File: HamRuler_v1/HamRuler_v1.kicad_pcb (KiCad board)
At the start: 2 copper layers, 13 parts, among them J1 Conn_01x03, Q1 BUK7M9R9-60EX, Q2 BUK7M9R9-60EX, U1 AT42QT1011-TSHR, U2 AT42QT1011-TSHR

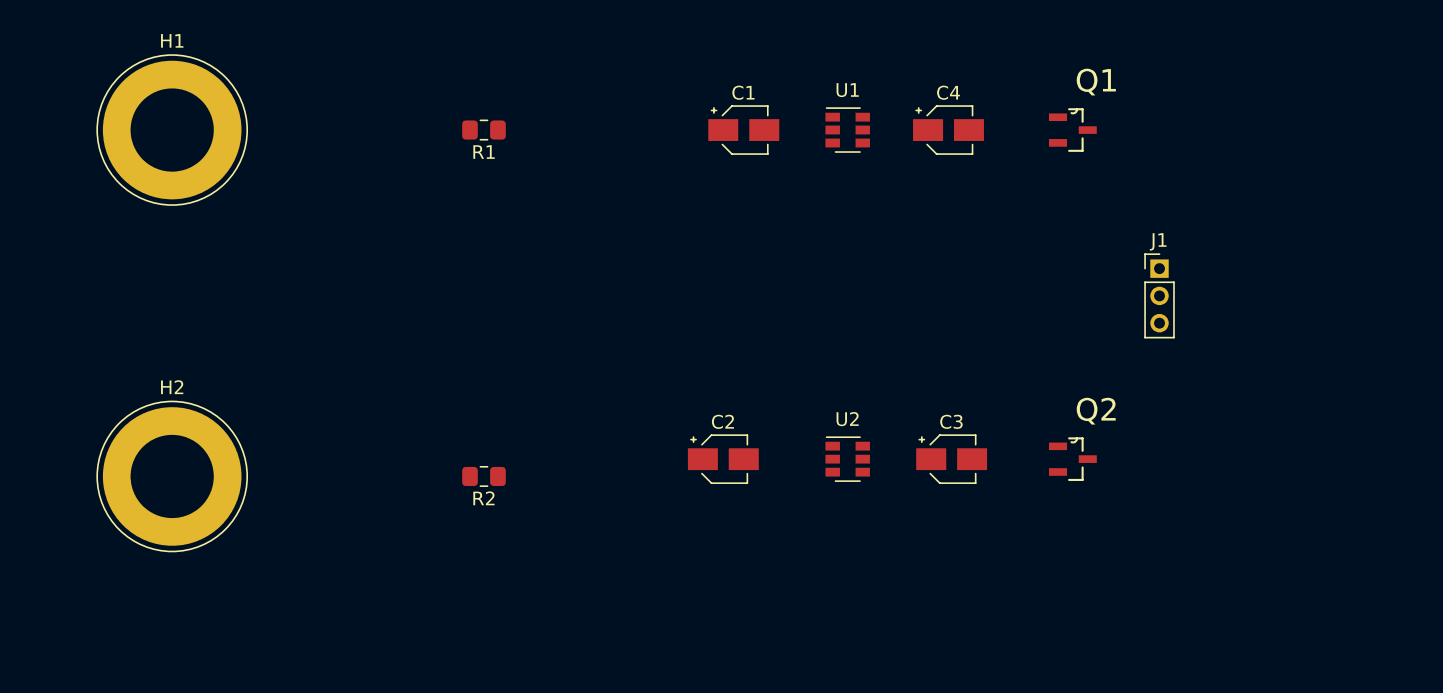
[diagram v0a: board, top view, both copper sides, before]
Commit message: nightly
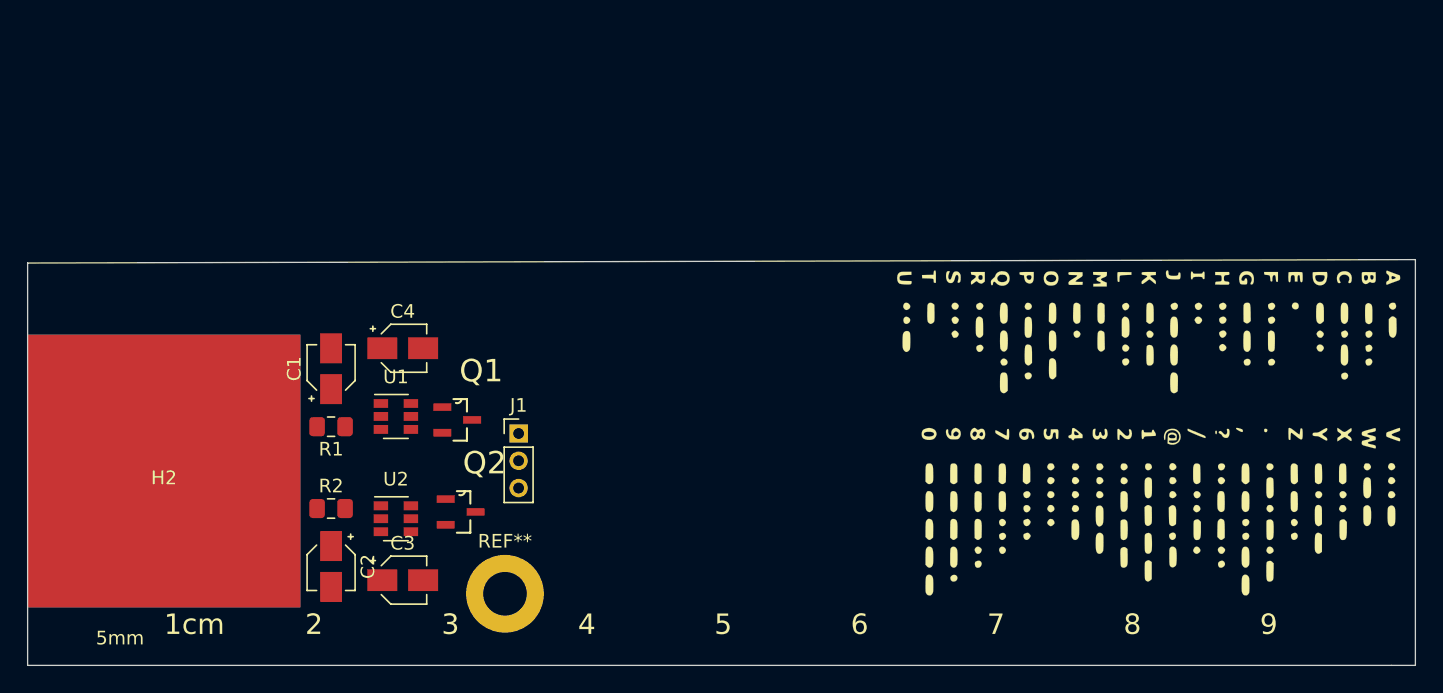
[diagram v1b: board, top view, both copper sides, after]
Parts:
- added G***: LOGO, Resources:morse_code, F.Cu at (110.0, 85.8)
- added REF**: MountingHole_3.2mm_M3_ISO7380_Pad, MountingHole:MountingHole_3.2mm_M3_ISO7380_Pad, F.Cu at (62.5, 97.5)
- added REF**: 4in_ruler, Resources:4in_ruler, B.Cu at (27.5, 73.2)
- added REF**: Metric_Ruler_100mm, Resources:Metric_Ruler_100mm, F.Cu at (27.5, 102.8)
- H1: footprint Connector:Banana_Jack_1Pin -> Resources:Large Pad; moved to B.Cu
- H2: footprint Connector:Banana_Jack_1Pin -> Resources:Large Pad
- moved Q1 49.9 mm to (59.0, 84.8)
- moved J1 48.5 mm to (63.5, 85.8)
- moved Q2 45.1 mm to (59.2, 91.5)
- moved C4 43.1 mm to (55.0, 79.5)
- moved C3 41.2 mm to (55.0, 96.5)
- moved U1 39.2 mm to (54.5, 84.5)
- moved C1 35.0 mm to (49.8, 81.0), turned to 90 degrees
- moved U2 33.4 mm to (54.5, 92.0)
- moved C2 29.8 mm to (49.8, 95.5), turned to 270 degrees
- moved H1 25.0 mm to (37.5, 88.5)
- moved R1 24.5 mm to (49.8, 85.2)
- moved R2 11.5 mm to (49.8, 91.2), turned to 0 degrees
- moved H2 0.72 mm to (37.5, 88.5)
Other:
- board outline added: 101.8 x 29.8 mm

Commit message: updated kicad version
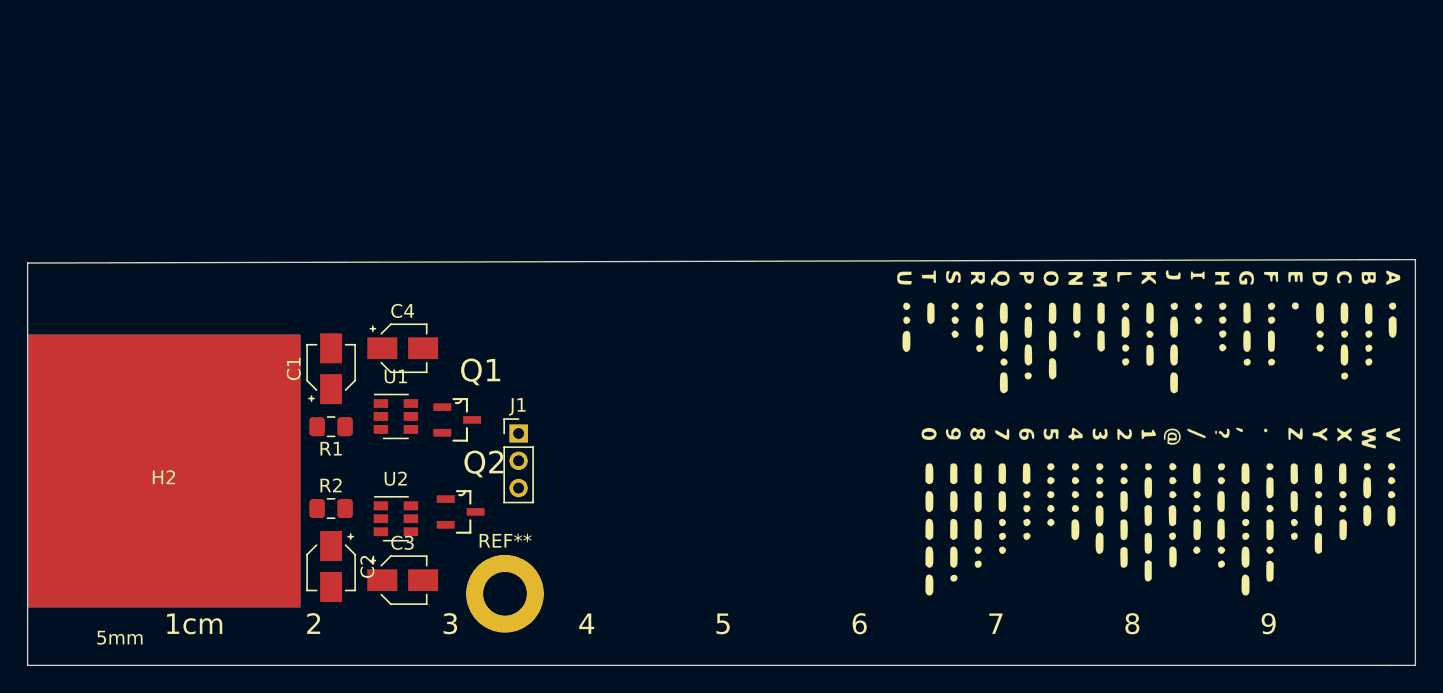
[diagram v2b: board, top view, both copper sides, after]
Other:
- net class Default removed

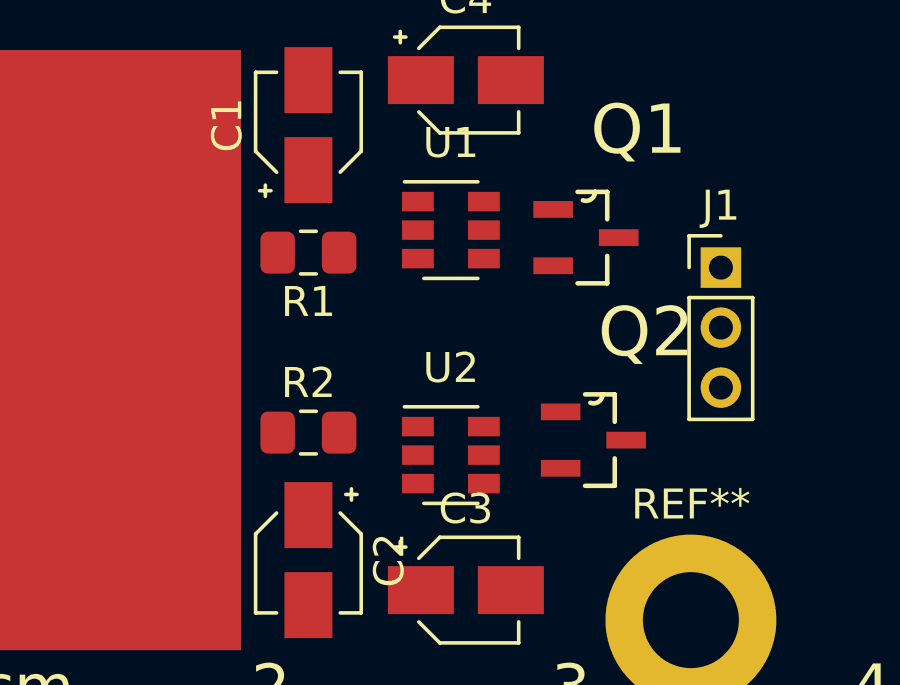
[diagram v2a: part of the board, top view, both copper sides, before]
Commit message: s
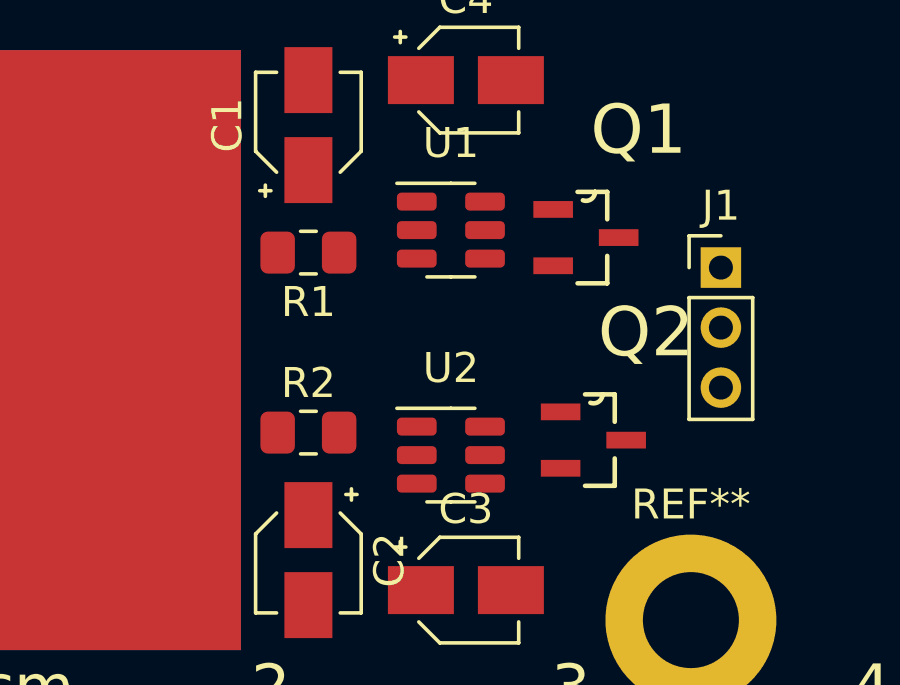
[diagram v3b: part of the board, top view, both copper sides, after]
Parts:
- added G***: LOGO, Resources:SELF_FULL_Stencil, B.Cu at (91.0, 93.0)
